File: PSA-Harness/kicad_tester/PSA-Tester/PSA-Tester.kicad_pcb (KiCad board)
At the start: 4 copper layers, 146 x 100 mm, 35 parts, among them J11 U262-241N-4BV60, SW1 B3S-1000, SW2 B3S-1000, SW3 B3S-1000, U1 MCP23017_SO, U10 ESP32-C3-OLED, U2 MCP23017_SO, U3 MCP23017_SO, U4 MCP23017_SO, U5 MCP23017_SO, U6 MCP23017_SO, U7 MCP23017_SO, U8 MCP23017_SO, U9 MCP23017_SO

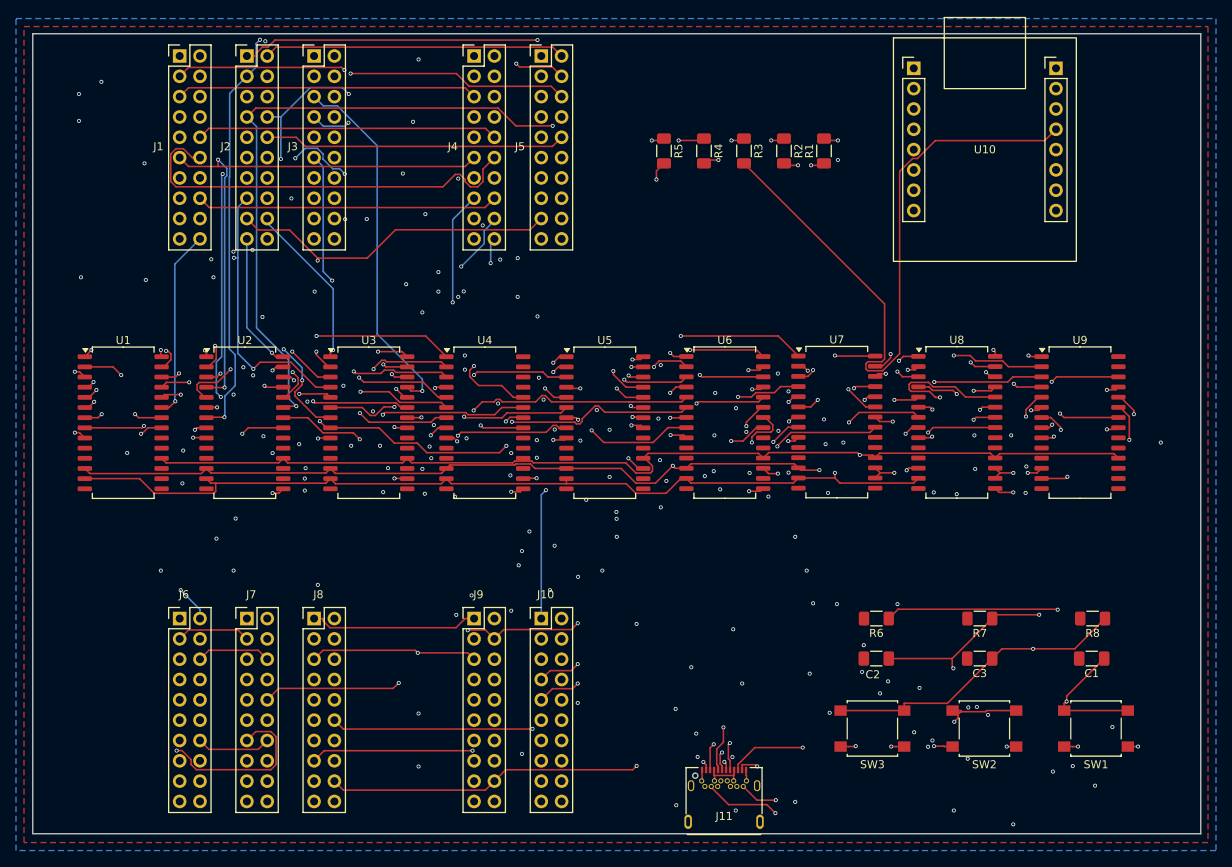
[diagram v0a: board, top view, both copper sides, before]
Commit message: 100x100mm routed
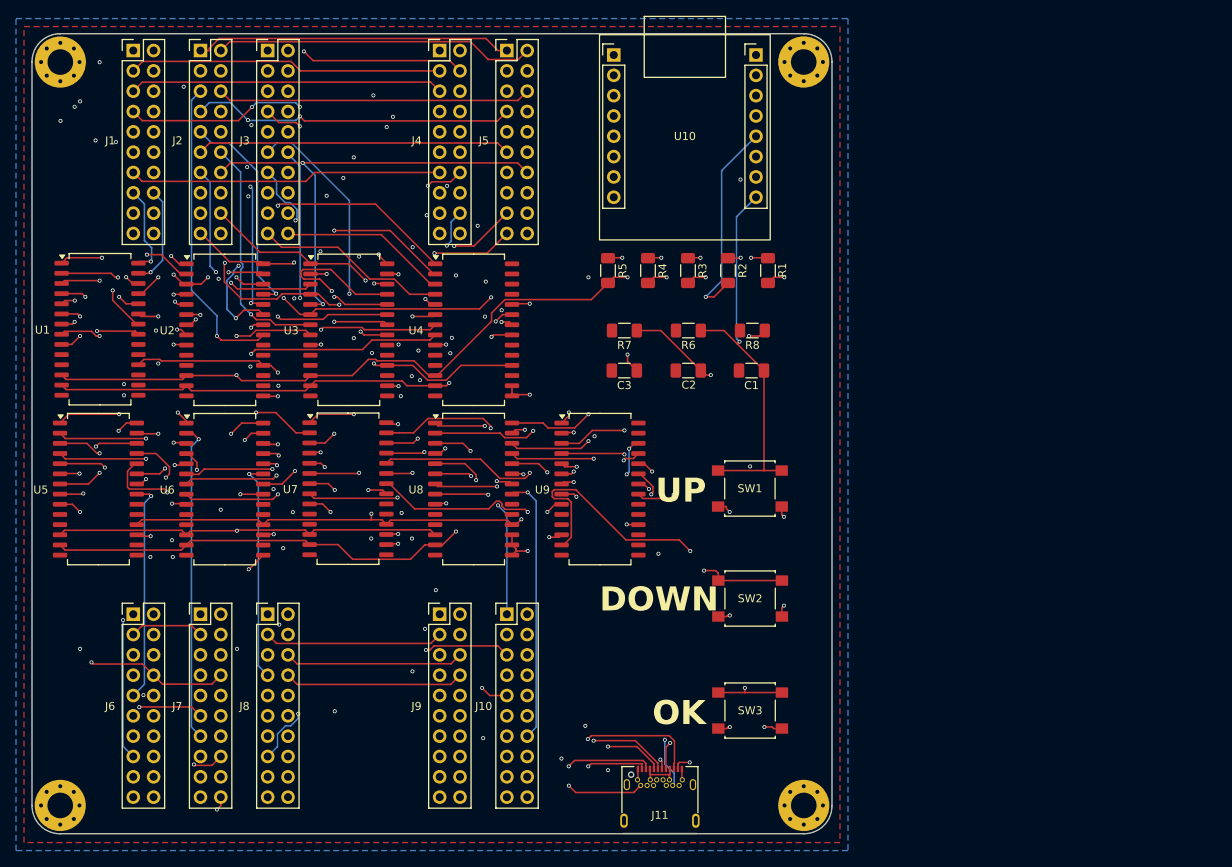
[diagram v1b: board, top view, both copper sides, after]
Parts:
- added M1: MountingHole_3.2mm_M3_Pad_Via, MountingHole:MountingHole_3.2mm_M3_Pad_Via, F.Cu at (42.5, 46.4)
- added M2: MountingHole_3.2mm_M3_Pad_Via, MountingHole:MountingHole_3.2mm_M3_Pad_Via, F.Cu at (135.5, 46.4)
- added M3: MountingHole_3.2mm_M3_Pad_Via, MountingHole:MountingHole_3.2mm_M3_Pad_Via, F.Cu at (42.5, 139.4)
- added M4: MountingHole_3.2mm_M3_Pad_Via, MountingHole:MountingHole_3.2mm_M3_Pad_Via, F.Cu at (135.5, 139.4)
- moved U5 63.8 mm to (47.3, 99.8)
- moved U6 63.1 mm to (63.1, 99.8)
- moved U7 61.7 mm to (78.5, 99.8)
- moved U8 61.0 mm to (94.2, 99.8)
- moved U9 60.6 mm to (110.0, 99.8)
- moved C3 57.2 mm to (113.0, 85.0)
- moved R7 57.2 mm to (113.0, 80.0)
- moved C1 55.7 mm to (128.9, 85.0)
- moved R8 55.7 mm to (129.1, 80.0)
- moved SW1 52.6 mm to (128.7, 99.8)
- moved R6 43.0 mm to (121.0, 80.0)
- moved C2 43.0 mm to (121.0, 85.0)
- moved U10 37.5 mm to (111.7, 45.6)
- moved SW2 33.5 mm to (128.8, 113.5)
- moved R1 16.5 mm to (131.0, 72.5)
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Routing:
- net 9a: track 128.0 -> 37.1 mm, vias 2 -> 1
- net 18a: track 134.4 -> 49.2 mm, vias 3 -> 1
- net 5a: track 108.3 -> 40.0 mm, vias 2 -> 1
- net 60a: track 105.6 -> 40.8 mm, vias 3 -> 1
- net 19a: track 109.4 -> 47.7 mm, vias 3 -> 1
- net 59a: track 92.3 -> 32.5 mm, vias 2 -> 1
- net 58a: track 94.1 -> 35.1 mm, vias 2 -> 1
- net 20a: track 100.8 -> 43.7 mm
- net 57a: track 90.0 -> 33.4 mm, vias 3 -> 1
- net 16a: track 109.1 -> 53.5 mm, vias 3 -> 2
- net 76: track 95.5 -> 40.5 mm, vias 3 -> 2
- net SCL2: track 131.7 -> 77.0 mm, vias 1 -> 3
- net 52a: track 102.3 -> 48.7 mm, vias 3 -> 1
- net 77: track 100.1 -> 48.0 mm, vias 2 -> 1
- net 7a: track 93.4 -> 41.9 mm, vias 3 -> 1
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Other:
- board size 146 x 100 mm -> 100 x 100 mm
- board text added: "DOWN"
- board text added: "OK"
- board text added: "UP"
